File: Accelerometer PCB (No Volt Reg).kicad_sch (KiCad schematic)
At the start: 21 parts, among them J1 S2B-PH-SM4-TB_LF__SN_, J2 M20-8770442, J3 MolexMicroSD, SW1 SW_Push, SW2 SW_Push, U1 Swan v3.0, U2 Sysrox Accelerometer, U3 Adafruit DS3231 RTC

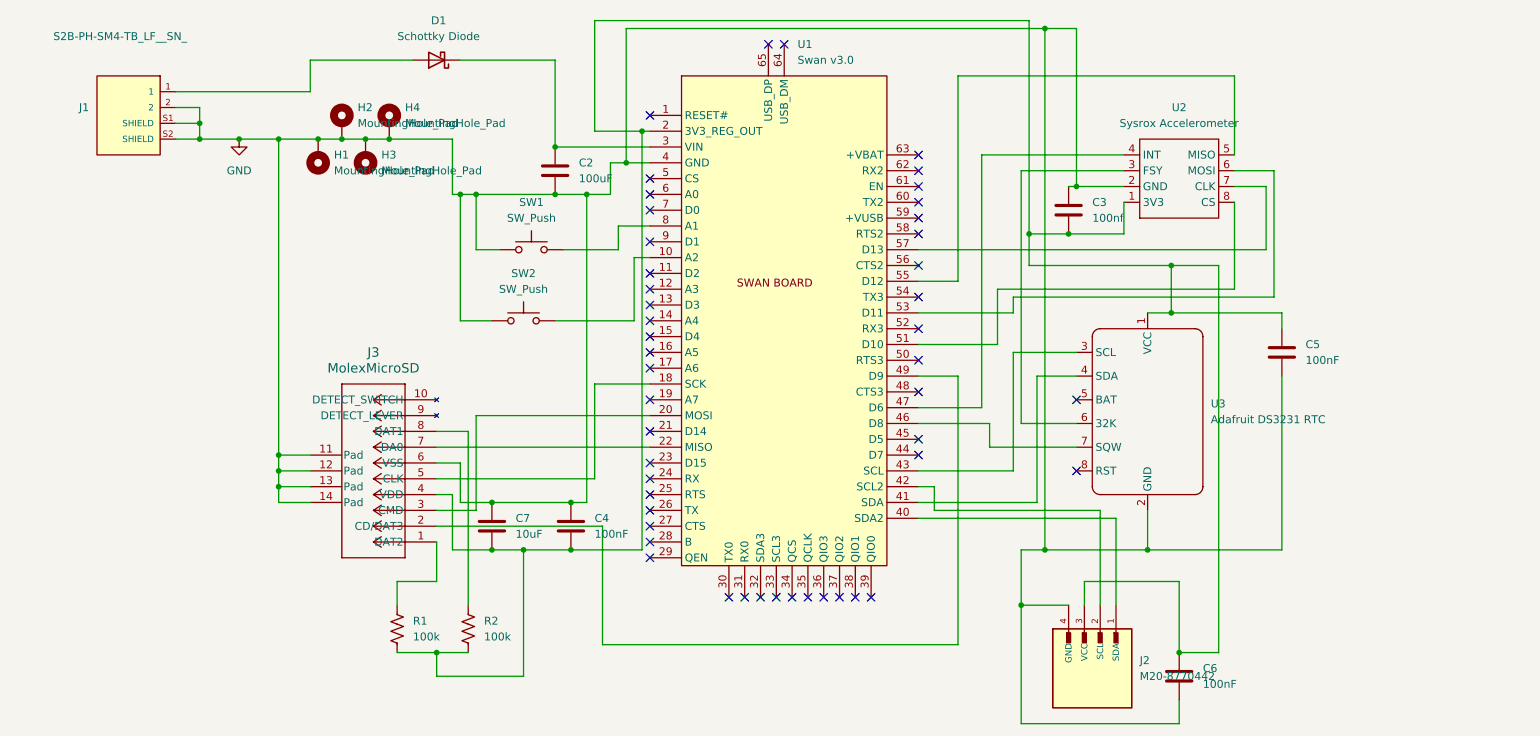
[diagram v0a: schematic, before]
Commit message: Add files via upload
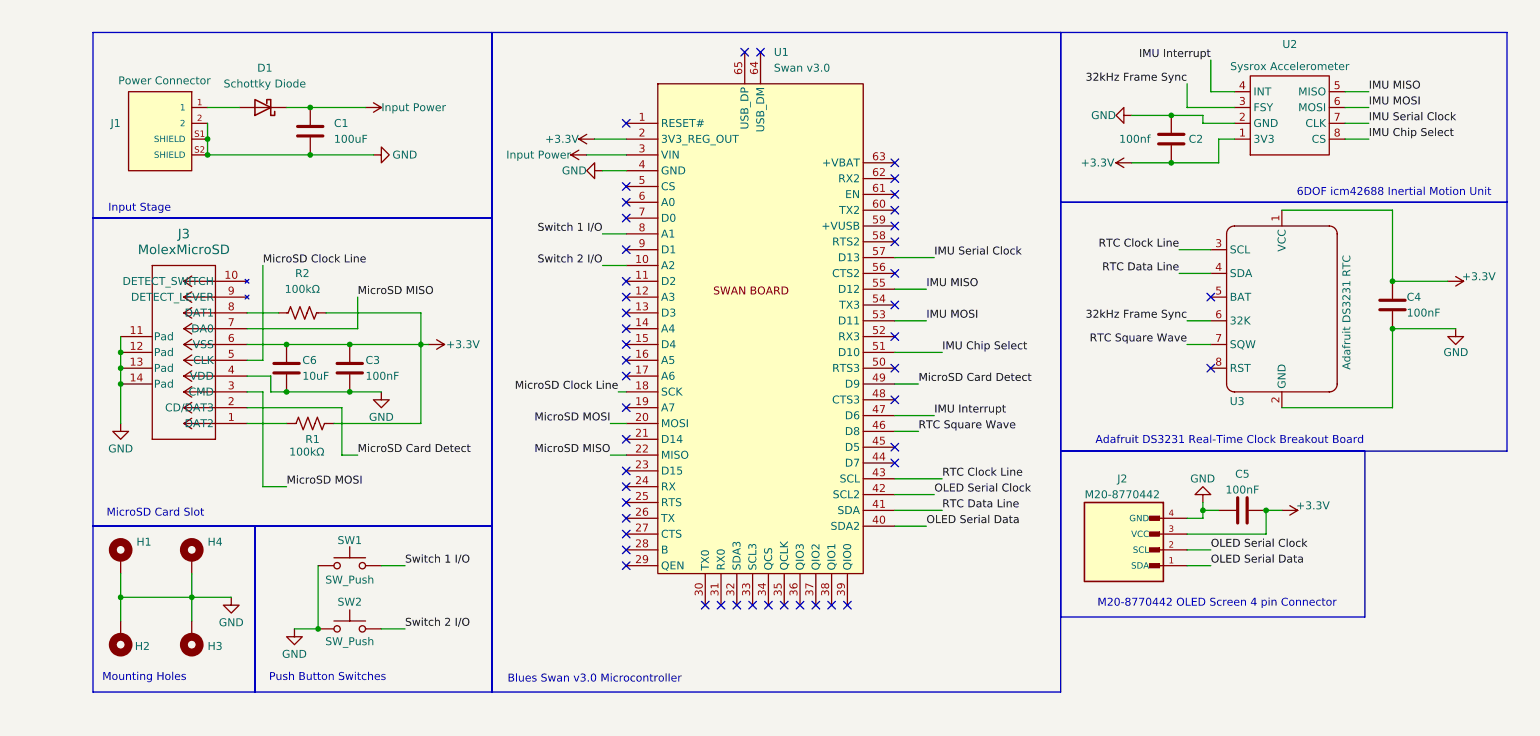
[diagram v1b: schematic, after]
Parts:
- removed C7: 10uF, Local Accelerometer Footprints:10uF External Input Cap, symbol Device:C
- added C1: 100uF, Local Accelerometer Footprints:BulkCap, symbol Device:C
- C2: value 100uF -> 100nf; footprint Local Accelerometer Footprints:BulkCap -> Local Accelerometer Footprints:Large Decoupling Capacitor
- C3: value 100nf -> 100nF
- C6: value 100nF -> 10uF; footprint Local Accelerometer Footprints:Large Decoupling Capacitor -> Local Accelerometer Footprints:10uF External Input Cap
- J1: value S2B-PH-SM4-TB_LF__SN_ -> Power Connector
- R1, R2: value 100k -> 100kΩ
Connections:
- net GND: now also C2.1, C3.2, C6.1, J3.4 (VDD), C1.2; no longer C2.2, C3.1, C6.2, J3.6 (VSS)
- net at J3.1 (DAT2): now also R1.2; no longer R1.1
- net +3.3V: now reaches C4.1, C5.1, J2.3 (VCC), R2.2, U1.2 (3V3_REG_OUT), U2.1 (3V3), U3.1 (VCC)
- net +3.3V: now also C2.2, C3.1, C6.2, J3.6 (VSS), R1.1; no longer C3.2, C6.1, J3.4 (VDD), R1.2
- net Input Power: now reaches D1.1 (K), U1.3 (VIN)
- net Input Power: now also C1.1; no longer C2.1
- net OLED Serial Data: now reaches J2.1 (SDA), U1.40 (SDA2)
- net OLED Serial Clock: now reaches J2.2 (SCL), U1.42 (SCL2)
- net Switch 2 I/O: now reaches SW2.2, U1.10 (A2)
- net 32kHz Frame Sync: now reaches U2.3 (FSY), U3.6 (32K)
- net IMU Interrupt: now reaches U1.47 (D6), U2.4 (INT)
- net IMU MISO: now reaches U1.55 (D12), U2.5 (MISO)
- net IMU MOSI: now reaches U1.53 (D11), U2.6 (MOSI)
- net IMU Serial Clock: now reaches U1.57 (D13), U2.7 (CLK)
- net IMU Chip Select: now reaches U1.51 (D10), U2.8 (CS)
- net MicroSD Clock Line: now reaches J3.5 (CLK), U1.18 (SCK)
- net MicroSD MOSI: now reaches J3.3 (CMD), U1.20 (MOSI)
- net MicroSD MISO: now reaches J3.7 (DA0), U1.22 (MISO)
- net RTC Data Line: now reaches U1.41 (SDA), U3.4 (SDA)
- net RTC Clock Line: now reaches U1.43 (SCL), U3.3 (SCL)
- net RTC Square Wave: now reaches U1.46 (D8), U3.7 (SQW)
- net MicroSD Card Detect: now reaches J3.2 (CD/DAT3), U1.49 (D9)
- net Switch 1 I/O: now reaches SW1.2, U1.8 (A1)
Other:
- note added: "6DOF icm42688 Inertial Motion Unit"
- note added: "Adafruit DS3231 Real-Time Clock Breakout Board"
- note added: "Blues Swan v3.0 Microcontroller"
- note added: "Input Stage"
- note added: "M20-8770442 OLED Screen 4 pin Connector"
- note added: "MicroSD Card Slot"
- note added: "Mounting Holes"
- note added: "Push Button Switches"
